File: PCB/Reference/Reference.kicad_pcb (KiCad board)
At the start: 2 copper layers, 70 x 70 mm, 28 parts, among them J1 Conn_01x04, U1 LMR16006XDDCR, U2 MD8942, U3 Barcode, U4 CH340X

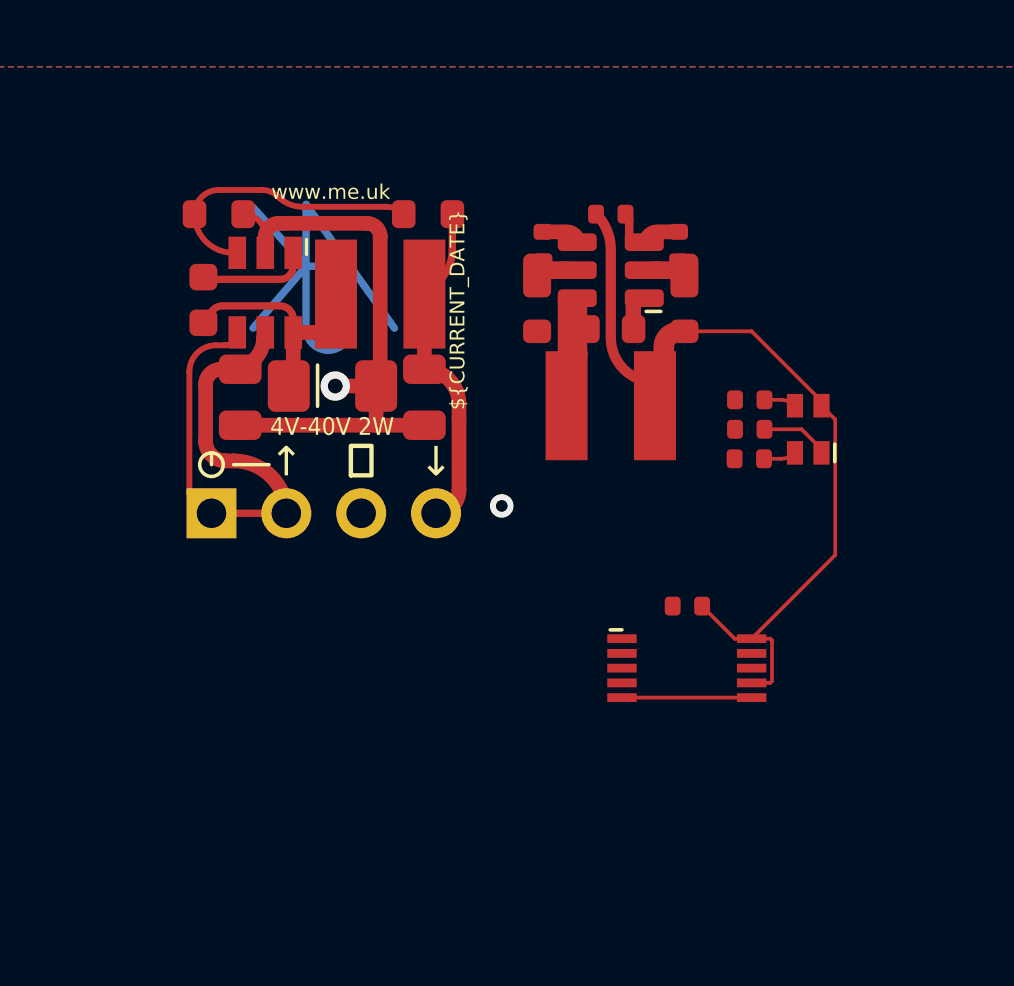
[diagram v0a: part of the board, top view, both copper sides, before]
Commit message: Fix RGB and tidy
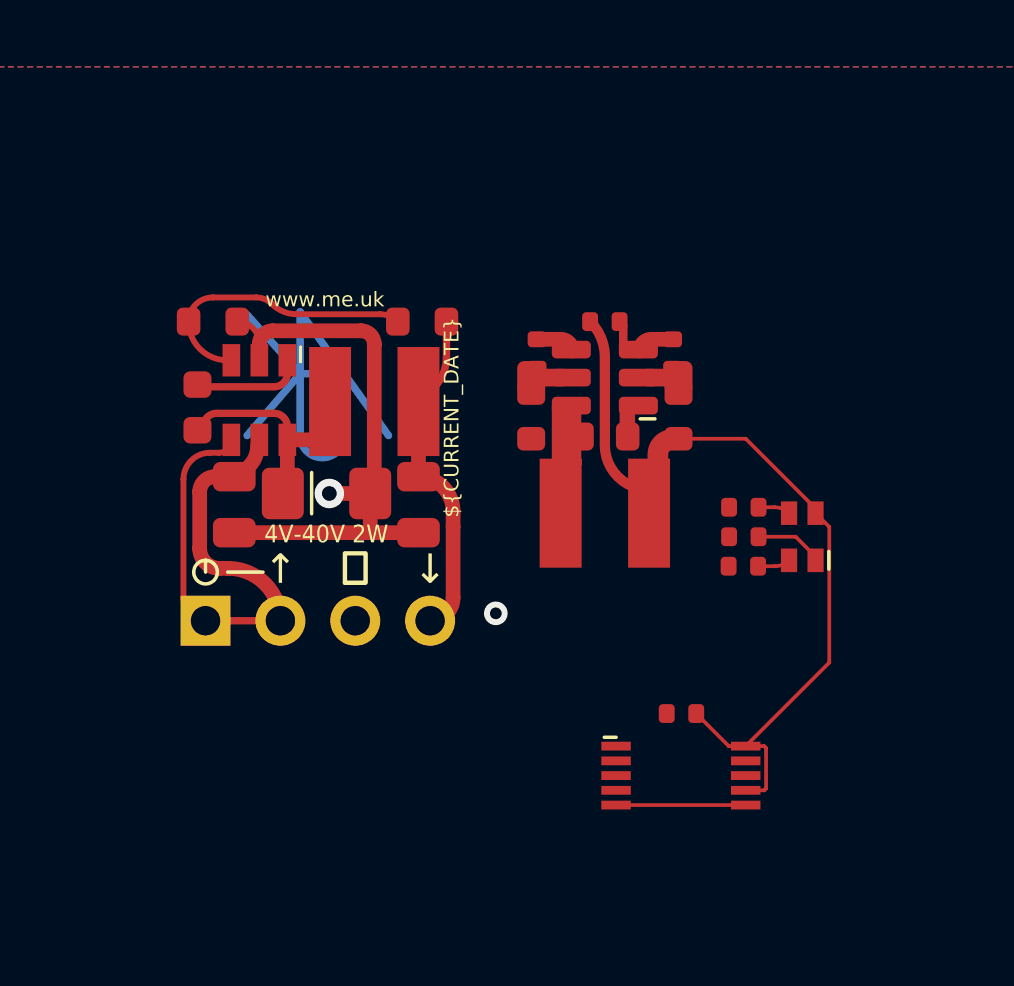
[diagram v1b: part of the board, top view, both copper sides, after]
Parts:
- moved C7 3.65 mm to (141.1, 58.9)
- moved J1 3.65 mm to (128.8, 55.8)
- moved Logo1 3.65 mm to (128.2, 47.4)
- moved C1 3.65 mm to (124.7, 48.6)
- moved R2 3.65 mm to (125.2, 45.6)
- moved C2 3.65 mm to (125.9, 51.9)
- moved C3 3.65 mm to (132.2, 51.9)
- moved C6 3.65 mm to (138.5, 49.5)
- moved D1 3.65 mm to (129.0, 51.5)
- moved D2 3.65 mm to (145.2, 52.9)
- moved L1 3.65 mm to (130.7, 48.3)
- moved L2 3.65 mm to (138.5, 52.1)
- moved R1 3.65 mm to (132.3, 45.6)
- moved R3 3.65 mm to (138.5, 45.6)
- moved R4 3.65 mm to (140.8, 46.7)
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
